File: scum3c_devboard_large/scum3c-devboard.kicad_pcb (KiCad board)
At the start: 2 copper layers, 39 x 72.9 mm, 59 parts, among them J1 CONSMA001-G, J10 Conn_01x02, J11 Conn_01x01, J2 47346-0001, J3 Conn_02x06_Odd_Even, J4 Conn_01x22, J5 Conn_02x04_Odd_Even, J6 Conn_01x03, J7 Conn_01x03, J8 Conn_01x03, J9 Conn_02x03_Odd_Even, U1 Perfboard, U10 74AVCH4T245D,118, U11 74AVCH4T245D,118, U12 S-85S1AB18-I6T1U, U13 74AVCH4T245D,118, U2 FT231XS-U, U3 74AVC1T45GS-Q100H, U4 74AVC1T45GS-Q100H, U5 ICM-20948, U6 S-85S1AB10-I6T1U, U7 S-85S1AB15-I6T1U, U8 scum3, U9 74AVCH4T245D,118

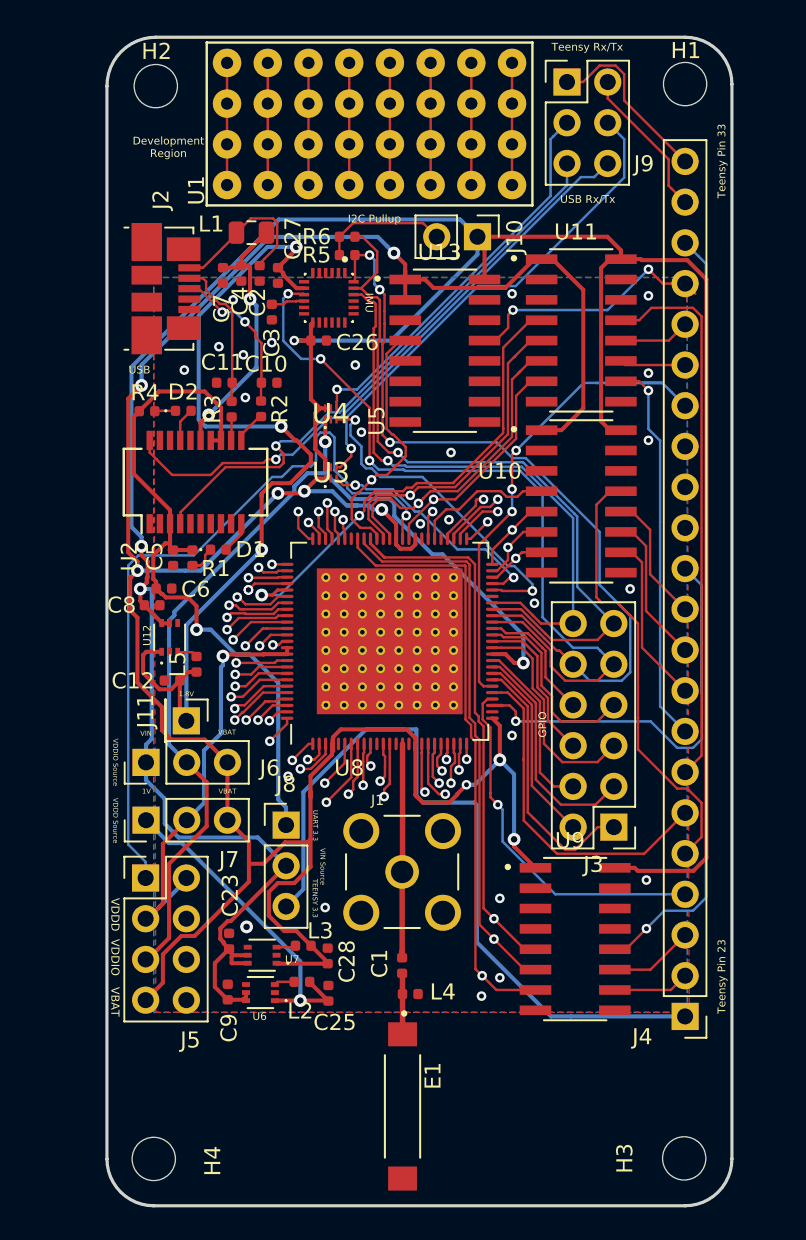
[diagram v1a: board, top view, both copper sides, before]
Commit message: Suggested changes
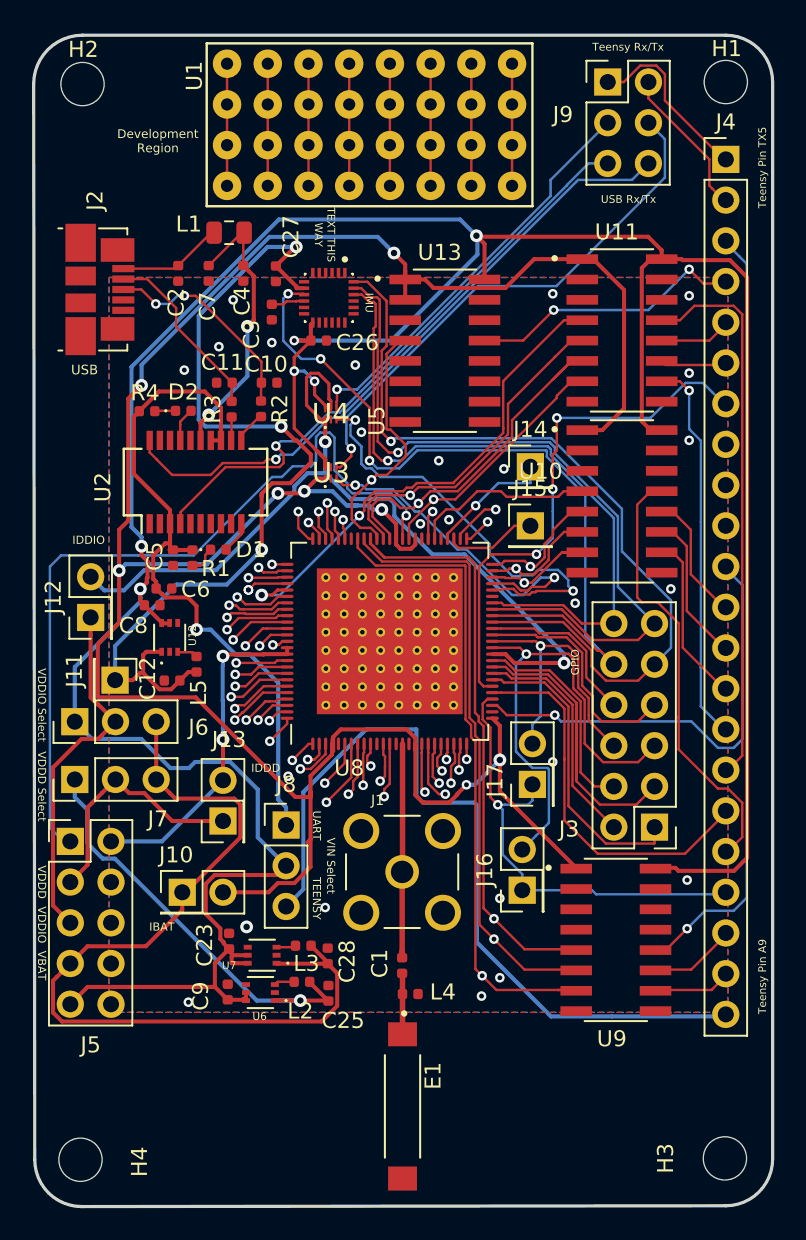
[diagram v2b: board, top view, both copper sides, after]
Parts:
- removed R5, R6: 10k, Resistor_SMD:R_0402_1005Metric
- added J12: Conn_02x01, Connector_PinHeader_2.54mm:PinHeader_2x01_P2.54mm_Vertical, F.Cu at (193.0, 103.5)
- added J13: Conn_02x01, Connector_PinHeader_2.54mm:PinHeader_2x01_P2.54mm_Vertical, F.Cu at (201.3, 116.2)
- added J14: Conn_01x01_Male, Connector_PinHeader_2.54mm:PinHeader_1x01_P2.54mm_Vertical, F.Cu at (220.5, 94.1)
- added J15: Conn_01x01_Male, Connector_PinHeader_2.54mm:PinHeader_1x01_P2.54mm_Vertical, F.Cu at (220.5, 97.8)
- added J16: Conn_02x01, Connector_PinHeader_2.54mm:PinHeader_2x01_P2.54mm_Vertical, F.Cu at (220.0, 120.5)
- added J17: Conn_02x01, Connector_PinHeader_2.54mm:PinHeader_2x01_P2.54mm_Vertical, F.Cu at (220.6, 113.9)
- J10: value Conn_01x02 -> Conn_02x01; footprint Connector_PinHeader_2.54mm:PinHeader_1x02_P2.54mm_Vertical -> Connector_PinHeader_2.54mm:PinHeader_2x01_P2.54mm_Vertical
- J4: footprint Connector_PinHeader_2.54mm:PinHeader_1x22_P2.54mm_Vertical -> SCUM:Teensy_Connector
- J5: value Conn_02x04_Odd_Even -> Conn_02x05_Odd_Even; footprint Connector_PinHeader_2.54mm:PinHeader_2x04_P2.54mm_Vertical -> Connector_PinHeader_2.54mm:PinHeader_2x05_P2.54mm_Vertical
- moved J4 53.5 mm to (232.7, 74.9), turned to 0 degrees
- moved J10 44.8 mm to (198.8, 120.7), turned to 0 degrees
- moved J5 5.23 mm to (191.8, 117.5)
- moved J7 5.12 mm to (192.0, 113.6)
- moved J6 5.12 mm to (192.0, 110.0)
- moved J11 5.12 mm to (194.6, 107.4)
- moved C2 5.08 mm to (198.5, 82.0)
- moved H2 4.57 mm to (192.5, 70.2)
- moved H4 4.57 mm to (192.4, 137.3)
- moved J2 4.12 mm to (193.6, 83.0)
- moved H1 2.54 mm to (232.7, 70.1)
- moved U9 2.54 mm to (225.8, 123.6)
- moved H3 2.54 mm to (232.6, 137.3)
- moved U10 2.54 mm to (226.2, 96.3)
- moved U11 2.54 mm to (226.2, 85.6)
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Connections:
- net /1Vin renamed +1VIN
- C28 pad 1: +VBAT -> +VBAT'
- J10 pad 1: +VIN -> +VBAT'
- J10 pad 2: Net-(J10-Pad2) -> +VBAT
- J5 pad 3: +VDDD -> +VDDD'
- J5 pad 5: +VDDIO -> +VDDIO'
- J5 pad 7: +VBAT -> +VBAT'
- J6 pad 2: +VDDIO -> +VDDIO'
- J6 pad 3: +VBAT -> +VBAT'
- J7 pad 2: +VDDD -> +VDDD'
- J7 pad 3: +VBAT -> +VBAT'
- L3 pad 1: +VBAT -> +VBAT'
- U1 pad 12: (no net) -> Net-(U1-Pad12)
- U1 pad 13: (no net) -> Net-(U1-Pad13)
- U1 pad 14: (no net) -> Net-(U1-Pad14)
- U1 pad 15: (no net) -> Net-(U1-Pad15)
- U1 pad 16: (no net) -> Net-(U1-Pad16)
- U1 pad 17: (no net) -> Net-(U1-Pad17)
- U1 pad 18: (no net) -> Net-(U1-Pad18)
- U1 pad 21: (no net) -> Net-(U1-Pad11)
- U1 pad 22: (no net) -> Net-(U1-Pad12)
- U1 pad 23: (no net) -> Net-(U1-Pad13)
- U1 pad 24: (no net) -> Net-(U1-Pad14)
- U1 pad 25: (no net) -> Net-(U1-Pad15)
- U1 pad 26: (no net) -> Net-(U1-Pad16)
- U1 pad 27: (no net) -> Net-(U1-Pad17)
- U1 pad 28: (no net) -> Net-(U1-Pad18)
- U1 pad 31: (no net) -> Net-(U1-Pad11)
- U1 pad 32: (no net) -> Net-(U1-Pad12)
- U1 pad 33: (no net) -> Net-(U1-Pad13)
- U1 pad 34: (no net) -> Net-(U1-Pad14)
- U1 pad 35: (no net) -> Net-(U1-Pad15)
- U1 pad 36: (no net) -> Net-(U1-Pad16)
- U1 pad 37: (no net) -> Net-(U1-Pad17)
- U1 pad 38: (no net) -> Net-(U1-Pad18)
- U1 pad 41: (no net) -> Net-(U1-Pad11)
- U1 pad 42: (no net) -> Net-(U1-Pad12)
- U1 pad 43: (no net) -> Net-(U1-Pad13)
- U1 pad 44: (no net) -> Net-(U1-Pad14)
- U1 pad 45: (no net) -> Net-(U1-Pad15)
- U1 pad 46: (no net) -> Net-(U1-Pad16)
- U1 pad 47: (no net) -> Net-(U1-Pad17)
- U1 pad 48: (no net) -> Net-(U1-Pad18)
- U4 pad 5: GND -> +VDDIO
- U5 pad 14: Net-(U5-Pad1) -> Net-(U5-Pad14)
- U5 pad 15: Net-(U5-Pad1) -> Net-(U5-Pad15)
- U5 pad 16: Net-(U5-Pad1) -> Net-(U5-Pad16)
- U5 pad 17: Net-(U5-Pad1) -> Net-(U5-Pad17)
- U5 pad 2: Net-(U5-Pad1) -> Net-(U5-Pad2)
- U5 pad 24: /GPIO13 -> /GPIO12
- U5 pad 3: Net-(U5-Pad1) -> Net-(U5-Pad3)
- U5 pad 4: Net-(U5-Pad1) -> Net-(U5-Pad4)
- U5 pad 5: Net-(U5-Pad1) -> Net-(U5-Pad5)
- U5 pad 6: Net-(U5-Pad1) -> Net-(U5-Pad6)
- U5 pad 9: /GPIO12 -> /GPIO13
- U7 pad 1: +VBAT -> +VBAT'
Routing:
- net (no net): track 61.0 -> 0.00 mm
- net +VBAT': track 0.00 -> 55.5 mm
- net +VIN: track 183.3 -> 206.4 mm, vias 3 -> 6
- net +VDDIO': track 0.00 -> 22.4 mm
- net /GPIO8: track 13.7 -> 30.8 mm, vias 0 -> 1
- net +VBAT: track 173.4 -> 157.6 mm, vias 9 -> 8
- net +VDDD': track 0.00 -> 15.3 mm
- net /GPIO9: track 9.71 -> 18.6 mm, vias 0 -> 1
- net +VDDIO: track 62.0 -> 53.5 mm
- net Net-(J10-Pad2): track 7.92 -> 0.00 mm
- net Net-(U1-Pad18): track 0.00 -> 7.62 mm
- net Net-(U1-Pad17): track 0.00 -> 7.62 mm
- net Net-(U1-Pad16): track 0.00 -> 7.62 mm
- net Net-(U1-Pad15): track 0.00 -> 7.62 mm
- net Net-(U1-Pad14): track 0.00 -> 7.62 mm
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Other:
- board size 39 x 72.9 mm -> 46.1 x 73.1 mm
- board text added: "IBAT"
- board text added: "IDDD"
- board text added: "IDDIO"
- board text added: "TEENSY"
- board text added: "TEXT THIS WAY"
- board text added: "Teensy Pin A9"
- board text added: "Teensy Pin TX5"
- board text added: "UART"
- board text added: "VDDD Select"
- board text added: "VDDIO Select"
- board text added: "VIN Select"
- board text removed: "1.8V"
- board text removed: "1V"
- board text removed: "I2C Pullup"
- board text removed: "TEENSY 3.3"
- board text removed: "Teensy Pin 23"
- board text removed: "Teensy Pin 33"
- board text removed: "UART 3.3"
- board text removed: "VDDD Source"
- board text removed: "VDDIO Source"
- board text removed: "VIN"
- board text removed: "VIN Source"
